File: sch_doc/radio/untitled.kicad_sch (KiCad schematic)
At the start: 31 parts

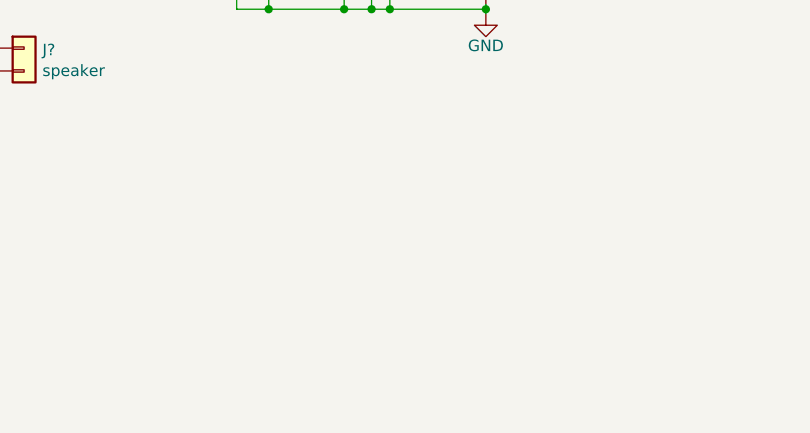
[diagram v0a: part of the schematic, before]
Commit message: new schematics, I hope that it will be final
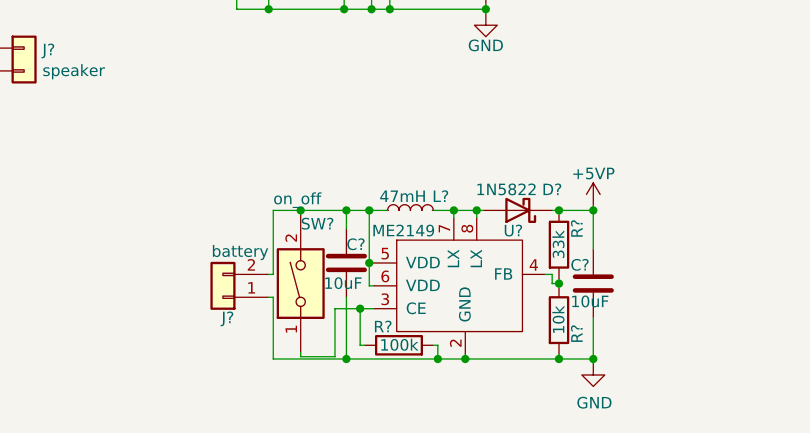
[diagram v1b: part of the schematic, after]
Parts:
- added C? (x2): 10uF, symbol Device:C
- added D?: 1N5822, Diode_THT:D_DO-201AD_P15.24mm_Horizontal, symbol Diode:1N5822
- added J?: battery, symbol Connector_Generic:Conn_01x02
- added L?: 47mH, Inductor_SMD:L_0603_1608Metric_Pad1.05x0.95mm_HandSolder, symbol tda:L
- added R?: 100k, symbol Device:R
- added R?: 33k, symbol Device:R
- added R?: 10k, symbol Device:R
- added SW?: on_off, symbol Switch:SW_DIP_x01
- added U?: ME2149, symbol local:ME2149
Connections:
- net GND: now also C?.1, C?.1, J?.1 (Pin_1), R?.2, R?.2, U?.2 (GND)
- new net: C?.2, J?.2 (Pin_2), L?.1, SW?.2, U?.5 (VDD), U?.6 (VDD)
- new net: R?.1, SW?.1, U?.3 (CE)
- new net: R?.1, R?.2, U?.4 (FB)
- new net: D?.2 (A), L?.2, U?.7 (LX), U?.8 (LX)
- new net +5VP: C?.2, D?.1 (K), R?.1
